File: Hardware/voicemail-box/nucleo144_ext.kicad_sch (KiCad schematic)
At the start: 3 parts, among them J6 Micro_SD_Card_Det1

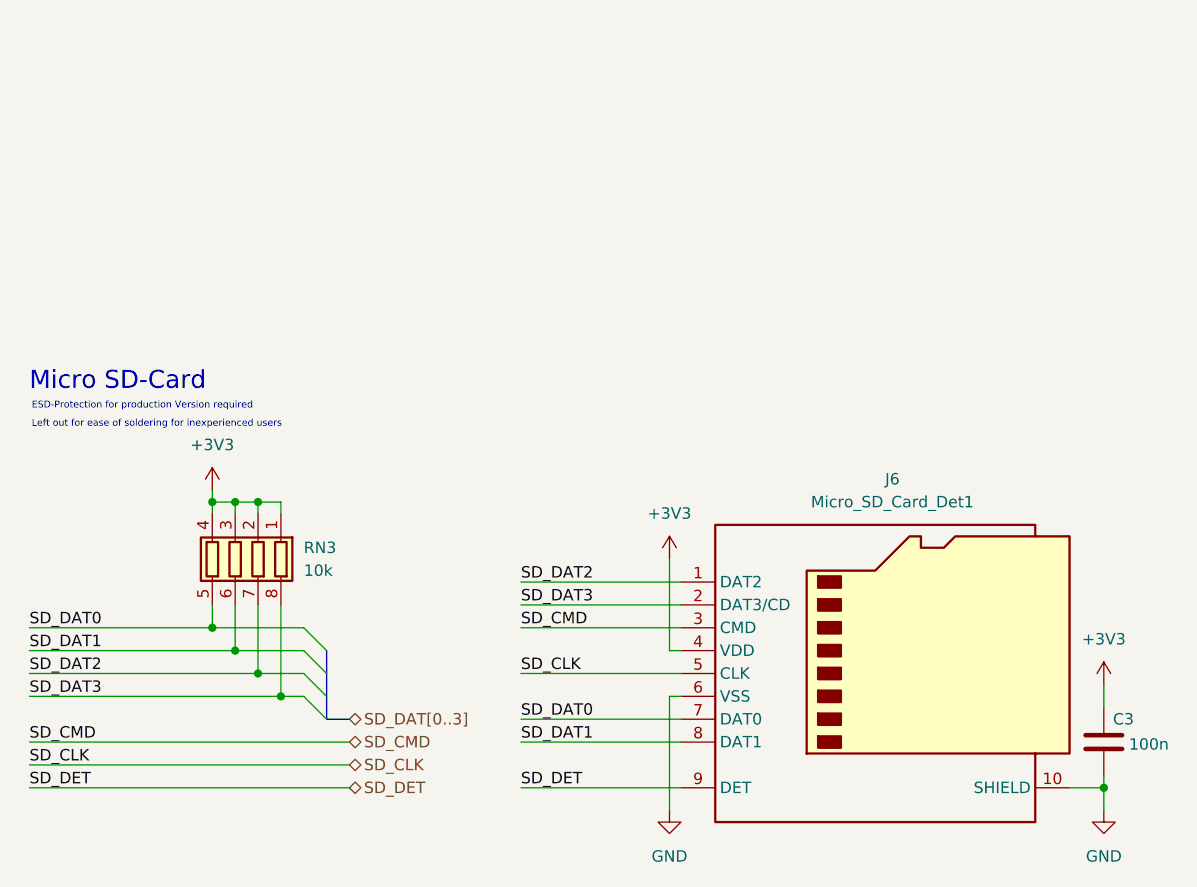
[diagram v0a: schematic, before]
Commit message: ~ HW Configuration
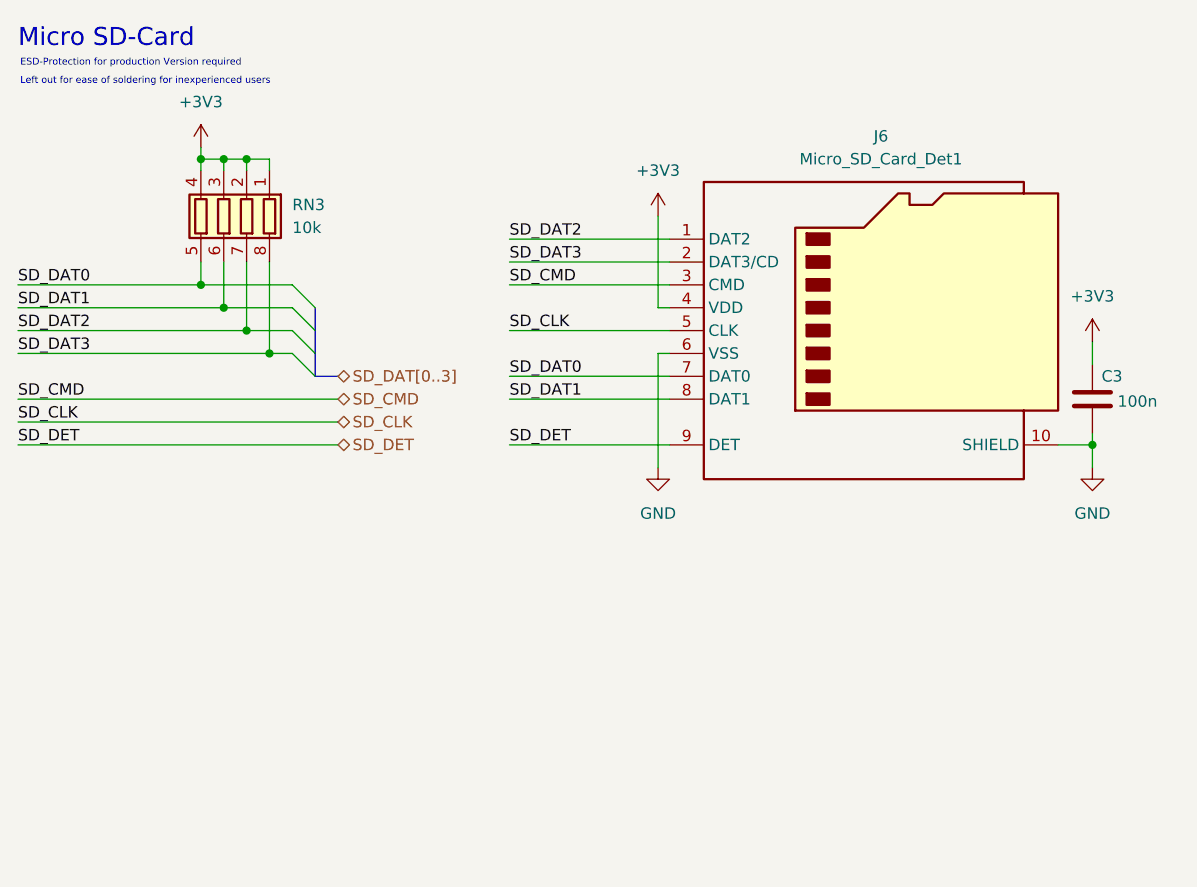
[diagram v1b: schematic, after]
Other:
- moved on the sheet: C3, J6, RN3

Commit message: ~working on first pcb-Draft
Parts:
- J6: footprint (none) -> Connector_Card:microSD_HC_Hirose_DM3AT-SF-PEJM5
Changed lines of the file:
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@@
 			)
 		)
-		(property "Footprint" ""
+		(property "Footprint" "Connector_Card:microSD_HC_Hirose_DM3AT-SF-PEJM5"
 			(at 166.37 34.29 0)
 			(effects
